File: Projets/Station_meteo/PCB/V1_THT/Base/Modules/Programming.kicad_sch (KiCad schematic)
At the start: 7 parts, among them J15 SolderJumper_2_Bridged, J16 SolderJumper_2_Bridged, J8 USB_C_Receptacle, U10 CH340G, Y2 12MHz

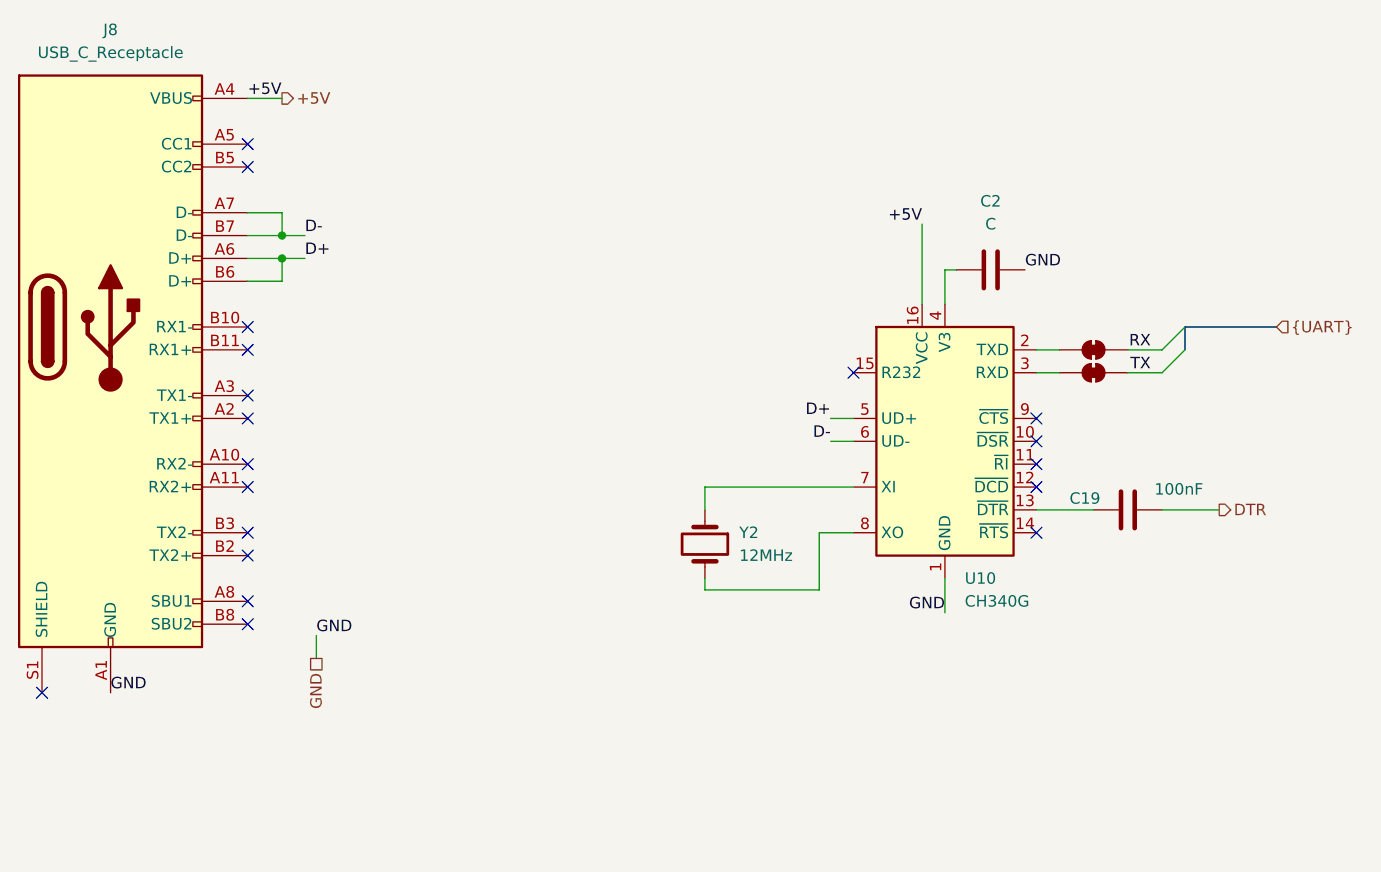
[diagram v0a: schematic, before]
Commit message: Update Weather station
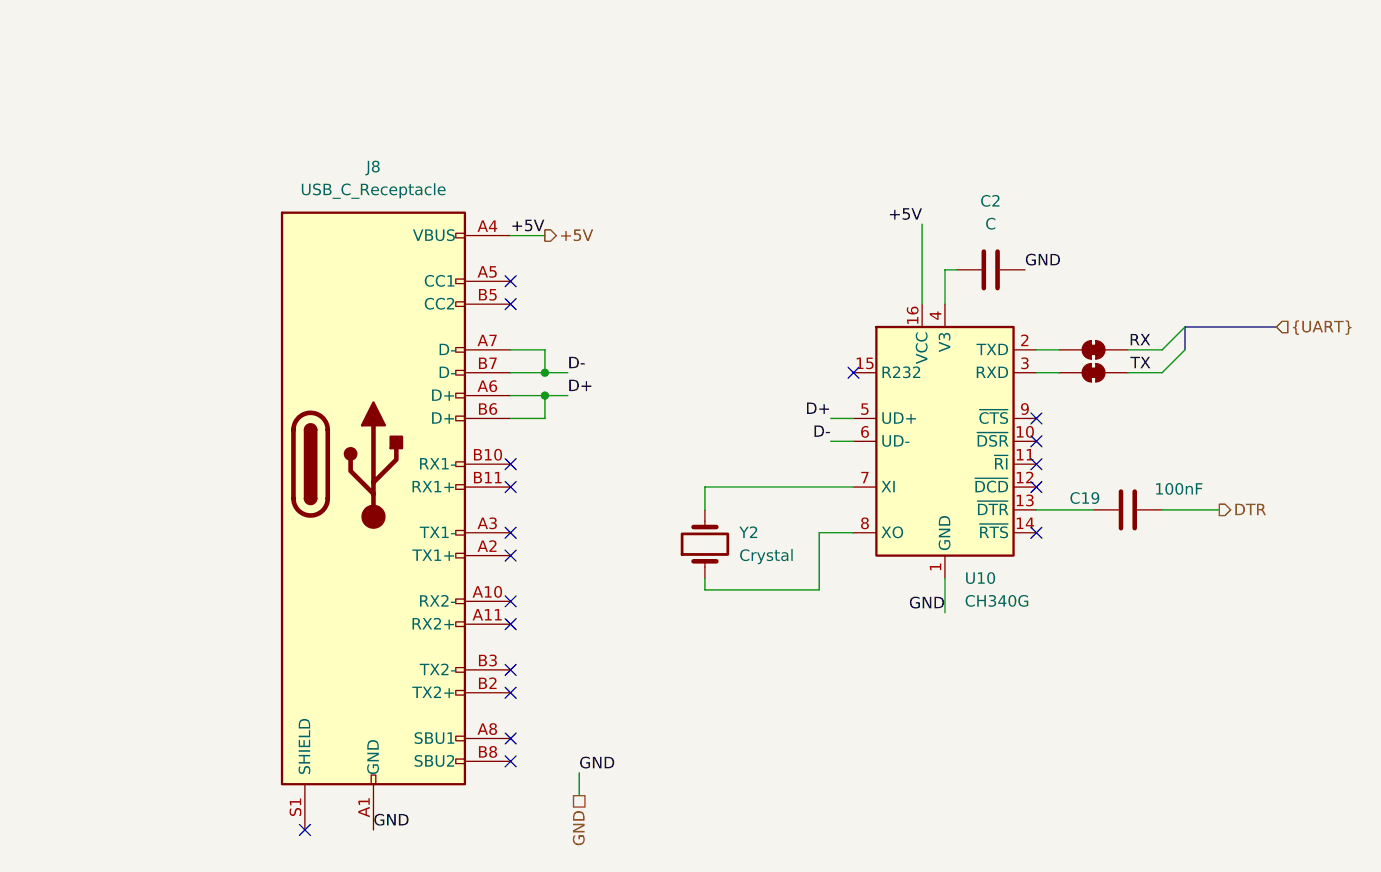
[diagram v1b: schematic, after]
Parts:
- Y2: value 12MHz -> Crystal; footprint Crystal:Crystal_SMD_HC49-SD -> Crystal:Crystal_HC49-4H_Vertical
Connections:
- net at U10.7 (XI): now also Y2.2; no longer Y2.1
- net at U10.8 (XO): now also Y2.1; no longer Y2.2
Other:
- moved on the sheet: J8
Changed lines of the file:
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@@
 	)
 	(junction
-		(at 19.05 44.45)
+		(at 48.26 59.69)
 		(diameter 0)
 		(color 0 0 0 0)
 	)
 	(junction
-		(at 19.05 41.91)
+		(at 48.26 57.15)
 		(diameter 0)
 		(color 0 0 0 0)
 	)
 	(no_connect
-		(at 15.24 31.75)
-	)
-	(no_connect
-		(at 15.24 77.47)
-	)
-	(no_connect
-		(at 15.24 54.61)
-	)
-	(no_connect
-		(at 15.24 62.23)
+		(at 44.45 46.99)
+	)
+	(no_connect
+		(at 44.45 92.71)
+	)
+	(no_connect
+		(at 44.45 69.85)
+	)
+	(no_connect
+		(at 44.45 77.47)
 	)
 	(no_connect
@@
 	)
 	(no_connect
-		(at -7.62 92.71)
+		(at 21.59 107.95)
 	)
 	(no_connect
@@
 	)
 	(no_connect
-		(at 15.24 69.85)
+		(at 44.45 85.09)
 	)
 	(no_connect
@@
 	)
 	(no_connect
-		(at 15.24 85.09)
-	)
-	(no_connect
-		(at 15.24 52.07)
-	)
-	(no_connect
-		(at 15.24 67.31)
-	)
-	(no_connect
-		(at 15.24 82.55)
+		(at 44.45 100.33)
+	)
+	(no_connect
+		(at 44.45 67.31)
+	)
+	(no_connect
+		(at 44.45 82.55)
+	)
+	(no_connect
+		(at 44.45 97.79)
 	)
 	(no_connect
@@
 	)
 	(no_connect
-		(at 15.24 74.93)
-	)
-	(no_connect
-		(at 15.24 34.29)
-	)
-	(no_connect
-		(at 15.24 59.69)
+		(at 44.45 90.17)
+	)
+	(no_connect
+		(at 44.45 49.53)
+	)
+	(no_connect
+		(at 44.45 74.93)
 	)
 	(no_connect
@@
 	(wire
 		(pts
-			(xy 15.24 46.99) (xy 19.05 46.99)
+			(xy 44.45 62.23) (xy 48.26 62.23)
 		)
 		(stroke
@@
 	(wire
 		(pts
-			(xy 19.05 44.45) (xy 19.05 46.99)
+			(xy 48.26 59.69) (xy 48.26 62.23)
 		)
 		(stroke
@@
 	(wire
 		(pts
-			(xy 19.05 39.37) (xy 19.05 41.91)
+			(xy 48.26 54.61) (xy 48.26 57.15)
 		)
 		(stroke
@@
 	(wire
 		(pts
-			(xy 19.05 41.91) (xy 21.59 41.91)
-		)
-		(stroke
-			(width 0)
-			(type default)
-		)
-	)
-	(wire
-		(pts
-			(xy 19.05 44.45) (xy 21.59 44.45)
+			(xy 48.26 57.15) (xy 50.8 57.15)
+		)
+		(stroke
+			(width 0)
+			(type default)
+		)
+	)
+	(wire
+		(pts
+			(xy 48.26 59.69) (xy 50.8 59.69)
 		)
 		(stroke
@@
 	(wire
 		(pts
-			(xy 15.24 44.45) (xy 19.05 44.45)
+			(xy 44.45 59.69) (xy 48.26 59.69)
 		)
 		(stroke
@@
 	(wire
 		(pts
-			(xy 15.24 39.37) (xy 19.05 39.37)
+			(xy 44.45 54.61) (xy 48.26 54.61)
 		)
 		(stroke
@@
 	(wire
 		(pts
-			(xy 15.24 26.67) (xy 19.05 26.67)
-		)
-		(stroke
-			(width 0)
-			(type default)
-		)
-	)
-	(wire
-		(pts
-			(xy 15.24 41.91) (xy 19.05 41.91)
-		)
-		(stroke
-			(width 0)
-			(type default)
-		)
-	)
-	(wire
-		(pts
-			(xy 22.86 86.36) (xy 22.86 88.9)
+			(xy 44.45 41.91) (xy 48.26 41.91)
+		)
+		(stroke
+			(width 0)
+			(type default)
+		)
+	)
+	(wire
+		(pts
+			(xy 44.45 57.15) (xy 48.26 57.15)
+		)
+		(stroke
+			(width 0)
+			(type default)
+		)
+	)
+	(wire
+		(pts
+			(xy 52.07 101.6) (xy 52.07 104.14)
 		)
 		(stroke
@@
 	)
 	(label "+5V"
-		(at 15.24 26.67 0)
+		(at 44.45 41.91 0)
 		(effects
 			(font
@@
 	)
 	(label "GND"
-		(at 22.86 86.36 0)
+		(at 52.07 101.6 0)
 		(effects
 			(font
@@
 	)
 	(label "D-"
-		(at 21.59 41.91 0)
+		(at 50.8 57.15 0)
 		(effects
 			(font
@@
 	)
 	(label "GND"
-		(at 0 92.71 0)
+		(at 29.21 107.95 0)
 		(effects
 			(font
@@
 	)
 	(label "D+"
-		(at 21.59 44.45 0)
+		(at 50.8 59.69 0)
 		(effects
 			(font
@@
 	(hierarchical_label "+5V"
 		(shape output)
-		(at 19.05 26.67 0)
+		(at 48.26 41.91 0)
 		(effects
 			(font
@@
 	(hierarchical_label "GND"
 		(shape passive)
-		(at 22.86 88.9 270)
+		(at 52.07 104.14 270)
 		(effects
 			(font
@@
 			)
 			(justify right)
-		)
-	)
-	(symbol
-		(lib_id "Device:Crystal")
-		(at 66.04 76.2 270)
-		(unit 1)
-		(exclude_from_sim no)
-		(in_bom yes)
-		(on_board yes)
-		(dnp no)
-		(fields_autoplaced yes)
-		(property "Reference" "Y2"
-			(at 69.85 74.9299 90)
-			(effects
-				(font
-					(size 1.27 1.27)
-				)
-				(justify left)
-			)
-		)
-		(property "Value" "12MHz"
-			(at 69.85 77.4699 90)
-			(effects
-				(font
-					(size 1.27 1.27)
-				)
-				(justify left)
-			)
-		)
-		(property "Footprint" "Crystal:Crystal_SMD_HC49-SD"
-			(at 66.04 76.2 0)
-			(effects
-				(font
-					(size 1.27 1.27)
-				)
-				(hide yes)
-			)
-		)
-		(property "Datasheet" "~"
-			(at 66.04 76.2 0)
-			(effects
-				(font
-					(size 1.27 1.27)
-				)
-				(hide yes)
-			)
-		)
-		(property "Description" "Two pin crystal"
-			(at 66.04 76.2 0)
-			(effects
-				(font
-					(size 1.27 1.27)
-				)
-				(hide yes)
-			)
-		)
-		(pin "2"
-		)
-		(pin "1"
-		)
-		(instances
-			(project "Weather"
-				(path "/4bc9f80e-0a24-4618-ba5d-3a118070c43e/d885458e-7b65-4bac-a9ac-9ebb78058802"
-					(reference "Y2")
-					(unit 1)
-				)
-			)
 		)
 	)
@@
 	)
 	(symbol
+		(lib_id "Device:Crystal")
+		(at 66.04 76.2 90)
+		(unit 1)
+		(exclude_from_sim no)
+		(in_bom yes)
+		(on_board yes)
+		(dnp no)
+		(fields_autoplaced yes)
+		(property "Reference" "Y2"
+			(at 69.85 74.9299 90)
+			(effects
+				(font
+					(size 1.27 1.27)
+				)
+				(justify right)
+			)
+		)
+		(property "Value" "Crystal"
+			(at 69.85 77.4699 90)
+			(effects
+				(font
+					(size 1.27 1.27)
+				)
+				(justify right)
+			)
+		)
+		(property "Footprint" "Crystal:Crystal_HC49-4H_Vertical"
+			(at 66.04 76.2 0)
+			(effects
+				(font
+					(size 1.27 1.27)
+				)
+				(hide yes)
+			)
+		)
+		(property "Datasheet" "~"
+			(at 66.04 76.2 0)
+			(effects
+				(font
+					(size 1.27 1.27)
+				)
+				(hide yes)
+			)
+		)
+		(property "Description" "Two pin crystal"
+			(at 66.04 76.2 0)
+			(effects
+				(font
+					(size 1.27 1.27)
+				)
+				(hide yes)
+			)
+		)
+		(pin "1"
+		)
+		(pin "2"
+		)
+		(instances
+			(project "Base"
+				(path "/4bc9f80e-0a24-4618-ba5d-3a118070c43e/d885458e-7b65-4bac-a9ac-9ebb78058802"
+					(reference "Y2")
+					(unit 1)
+				)
+			)
+		)
+	)
+	(symbol
 		(lib_id "CREPP_Connectors_USB_C:USB_C_Receptacle")
-		(at 0 52.07 0)
+		(at 29.21 67.31 0)
 		(unit 1)
 		(exclude_from_sim no)
@@
 		(fields_autoplaced yes)
 		(property "Reference" "J8"
-			(at 0 19.05 0)
+			(at 29.21 34.29 0)
 			(effects
 				(font
@@
 		)
 		(property "Value" "USB_C_Receptacle"
-			(at 0 21.59 0)
+			(at 29.21 36.83 0)
 			(effects
 				(font
@@
 		)
 		(property "Footprint" "CREPP_Connectors_USB:USB_C_Receptacle_GCT_USB4085"
-			(at 3.81 52.07 0)
+			(at 33.02 67.31 0)
 			(effects
 				(font
@@
 		)
 		(property "Datasheet" "https://www.usb.org/sites/default/files/documents/usb_type-c.zip"
-			(at 3.81 52.07 0)
+			(at 33.02 67.31 0)
 			(effects
 				(font
@@
 		)
 		(property "Description" "USB Full-Featured Type-C Receptacle connector"
-			(at 0 52.07 0)
-			(effects
-				(font
+			(at 29.21 67.31 0)
+			(effects
+				(font
